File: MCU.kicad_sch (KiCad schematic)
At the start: 0 parts

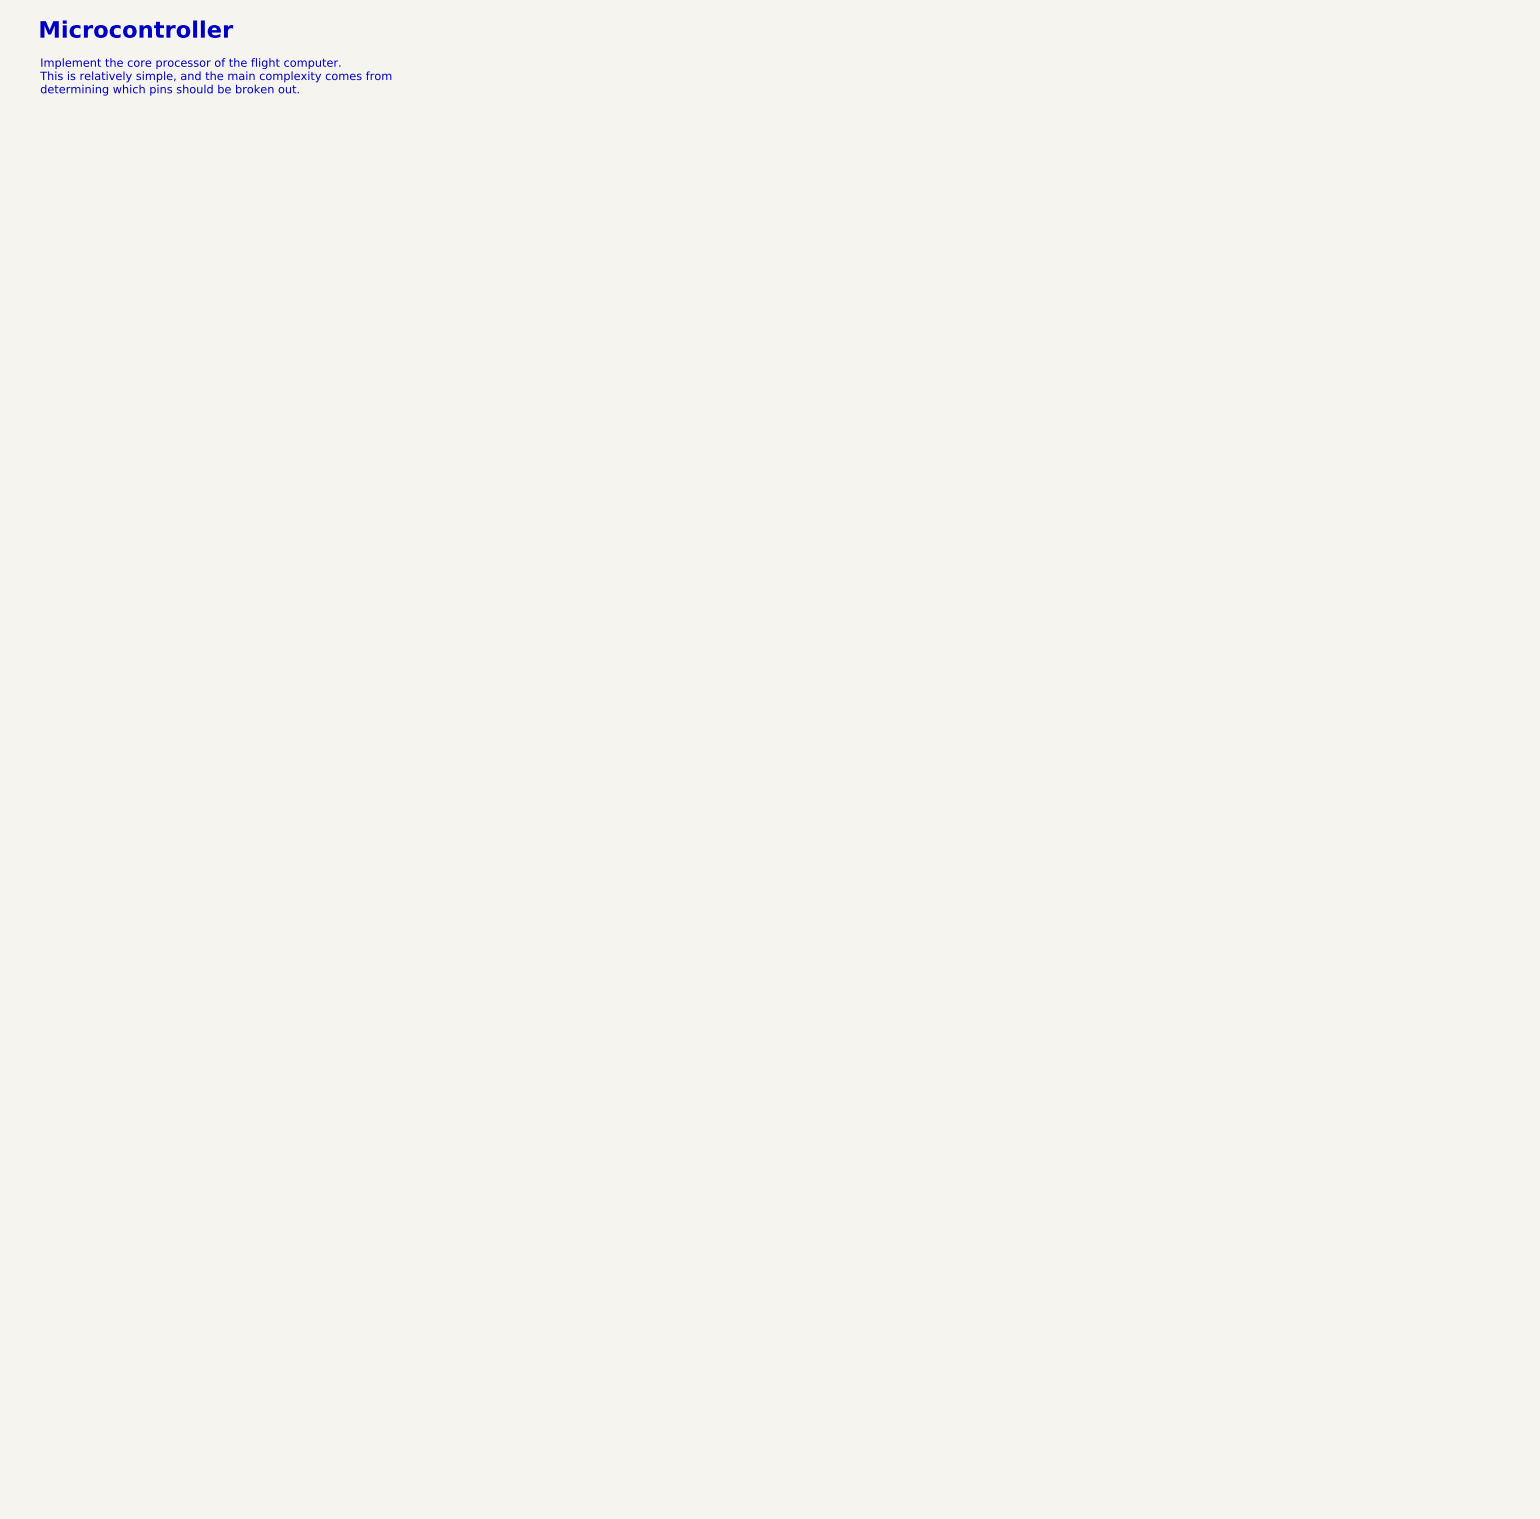
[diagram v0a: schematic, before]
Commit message: test
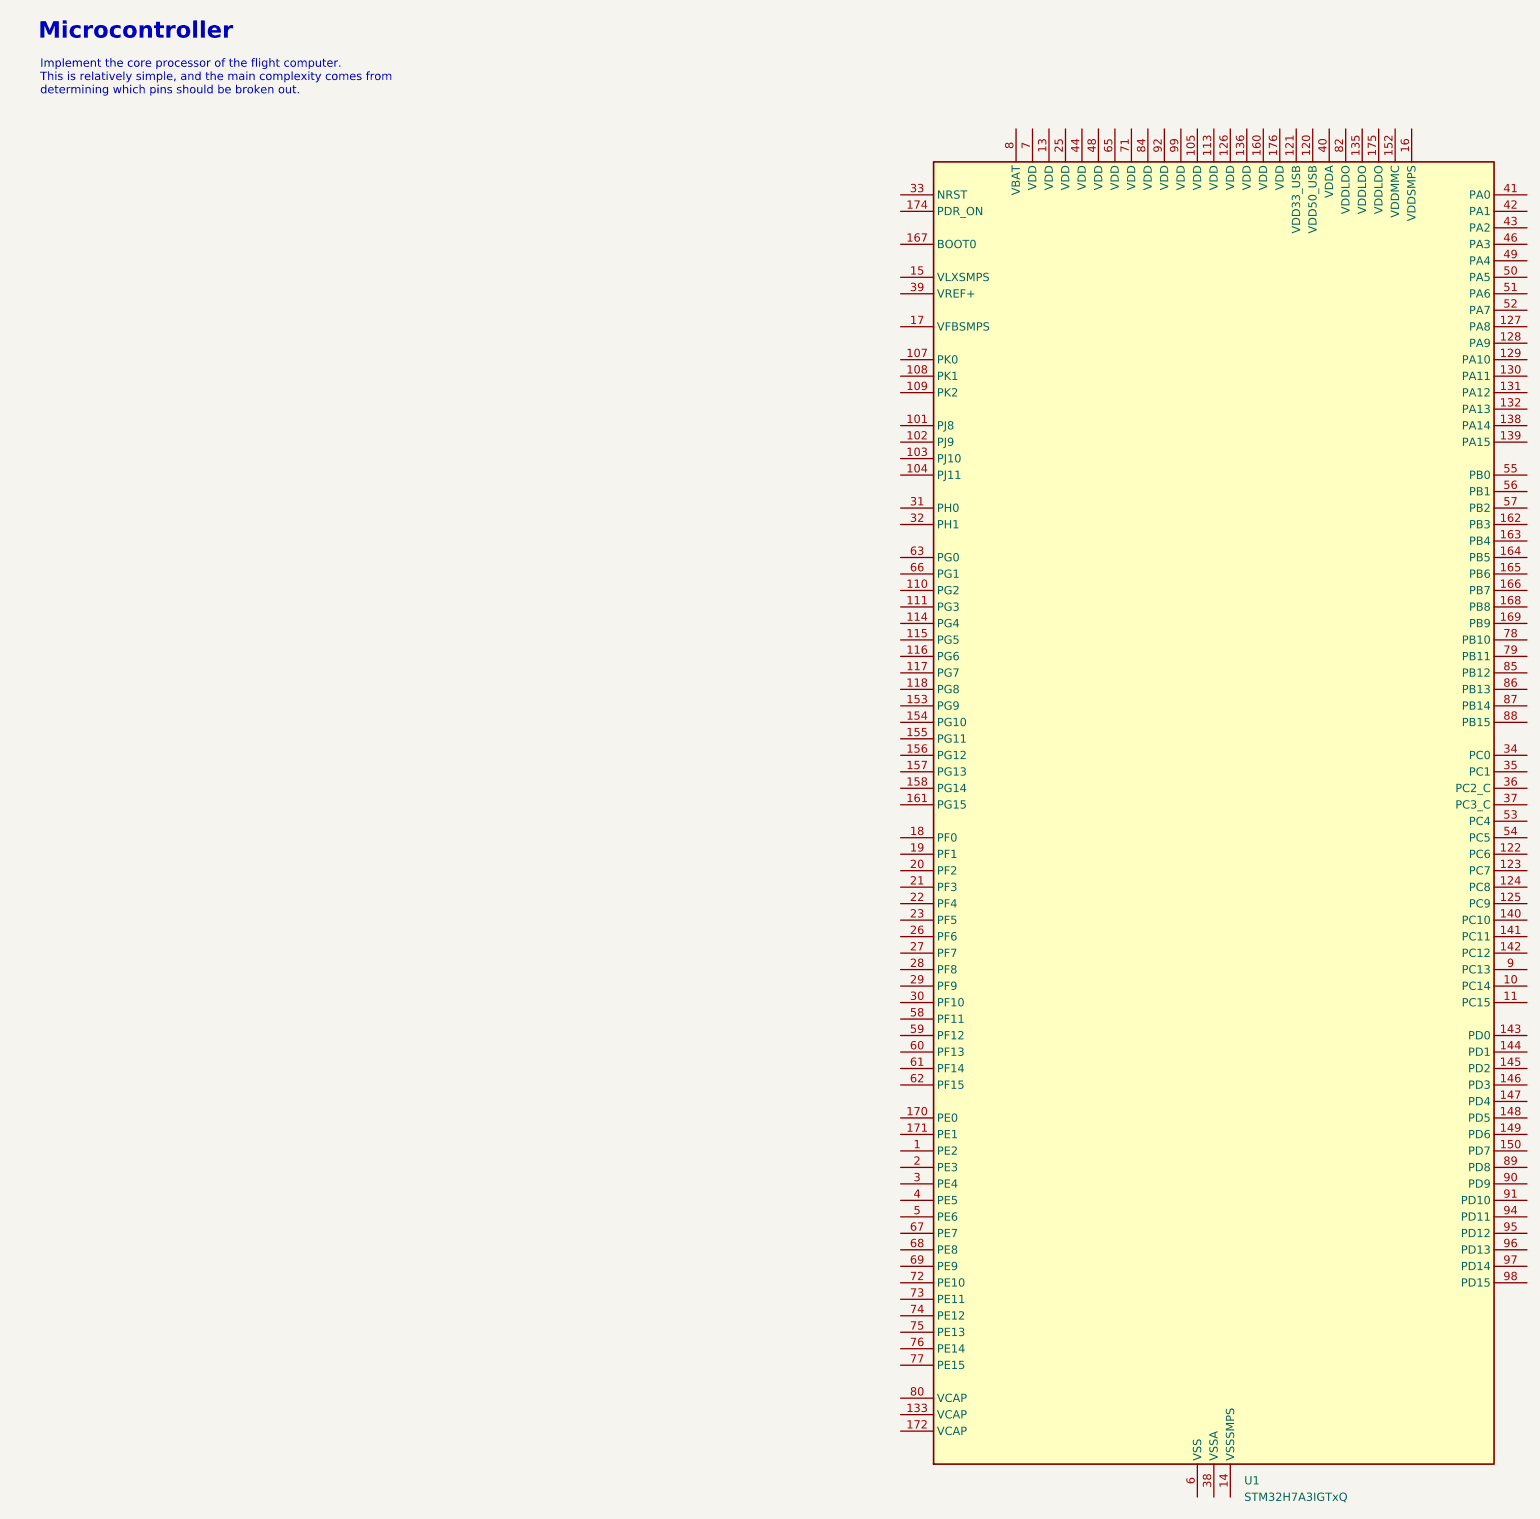
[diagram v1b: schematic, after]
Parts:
- added U1: STM32H7A3IGTxQ, Package_QFP:LQFP-176_24x24mm_P0.5mm, symbol MCU_ST_STM32H7:STM32H7A3IGTxQ
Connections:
- new net: U1.100 (VSS), U1.106 (VSS), U1.112 (VSS), U1.119 (VSS), U1.12 (VSS), U1.134 (VSS), U1.137 (VSS), U1.151 (VSS), U1.159 (VSS), U1.173 (VSS), U1.24 (VSS), U1.45 (VSS), U1.47 (VSS), U1.6 (VSS), U1.64 (VSS), U1.70 (VSS), U1.81 (VSS), U1.83 (VSS), U1.93 (VSS)

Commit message: renew
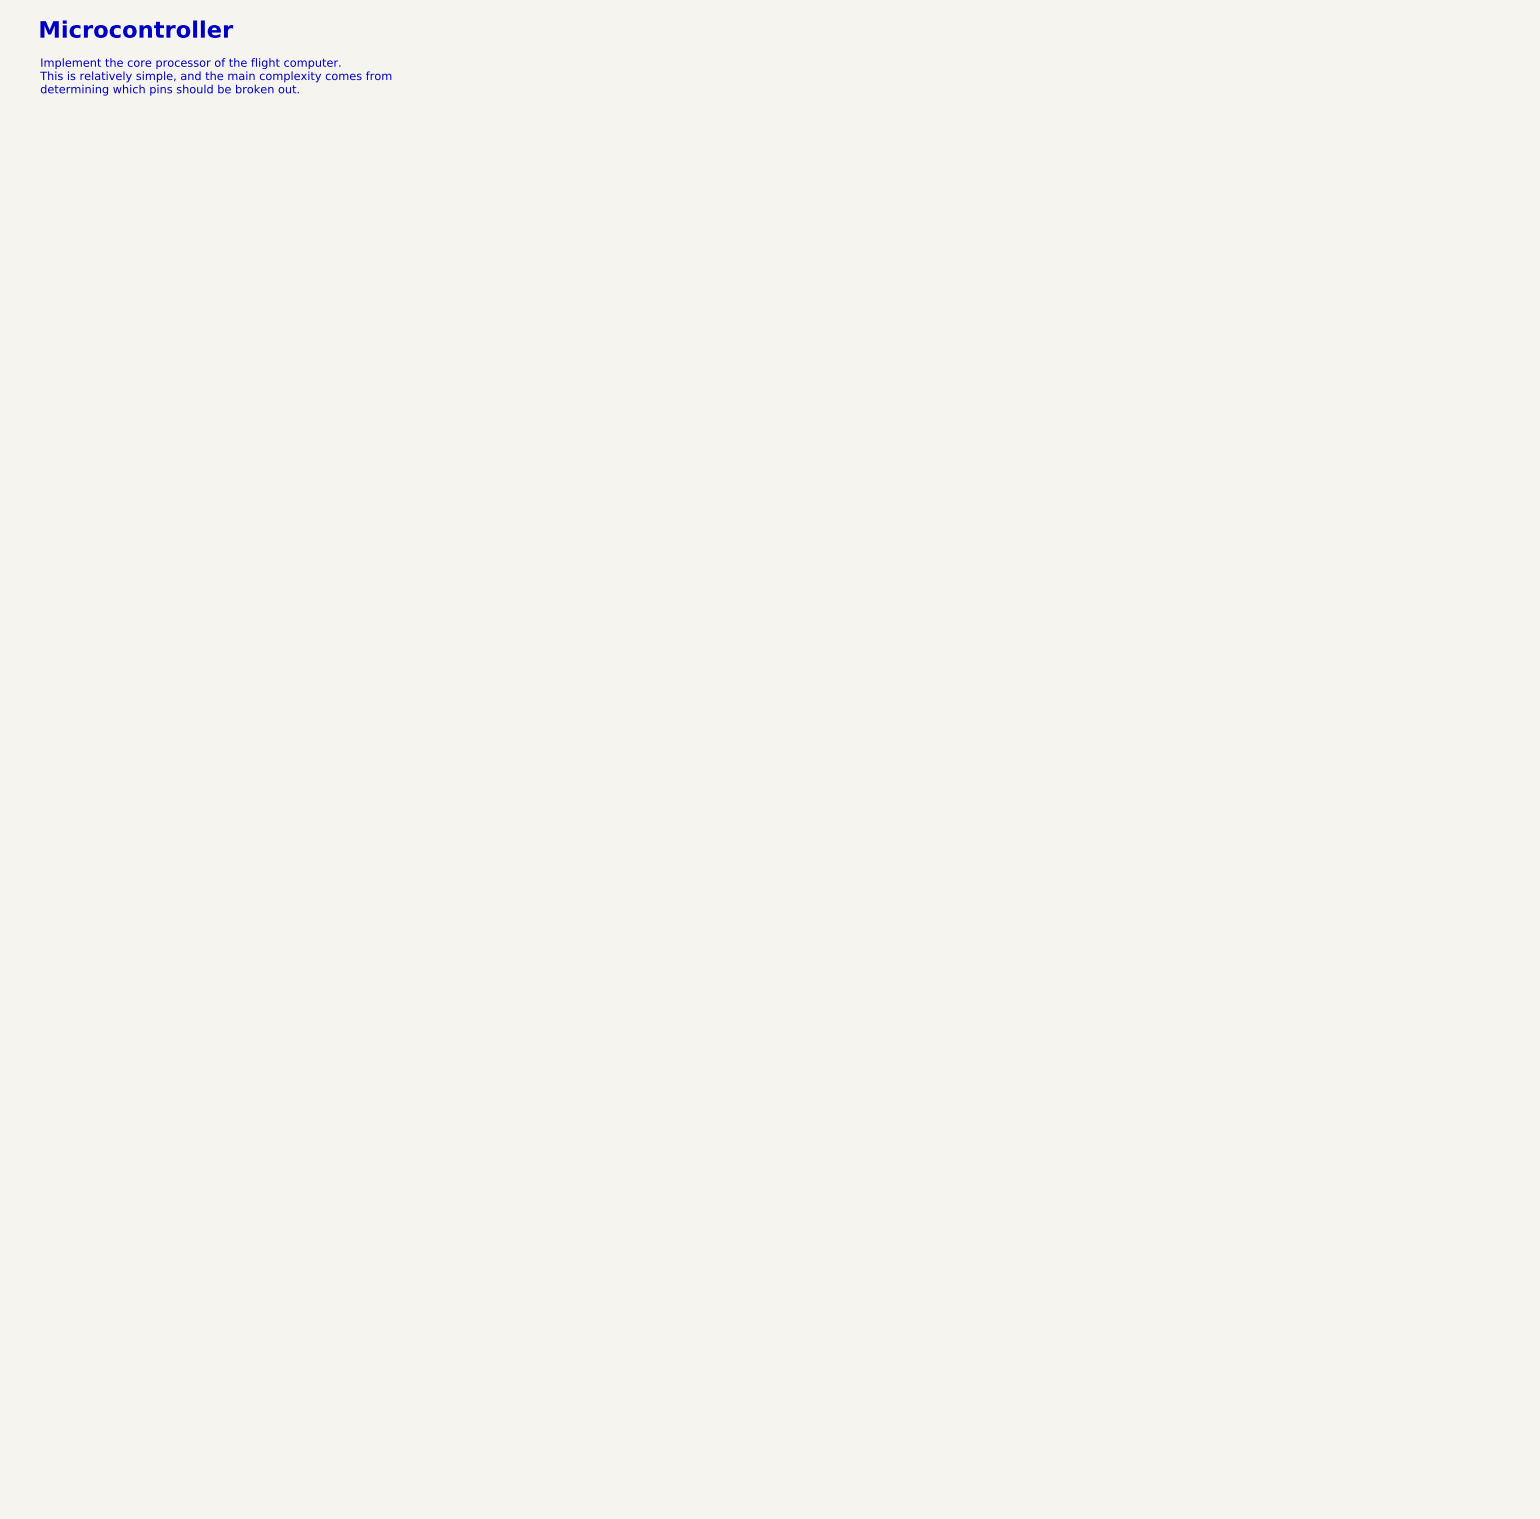
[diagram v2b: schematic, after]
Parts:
- removed U1: STM32H7A3IGTxQ, Package_QFP:LQFP-176_24x24mm_P0.5mm, symbol MCU_ST_STM32H7:STM32H7A3IGTxQ
